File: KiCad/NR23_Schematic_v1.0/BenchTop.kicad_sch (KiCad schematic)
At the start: 13 parts, among them M1 Zero_7R_Motor

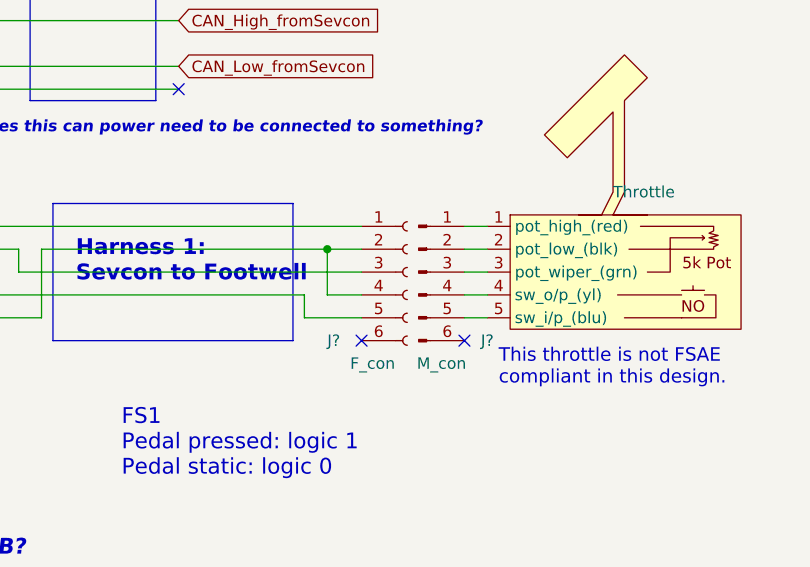
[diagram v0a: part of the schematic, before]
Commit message: Base update (V3)
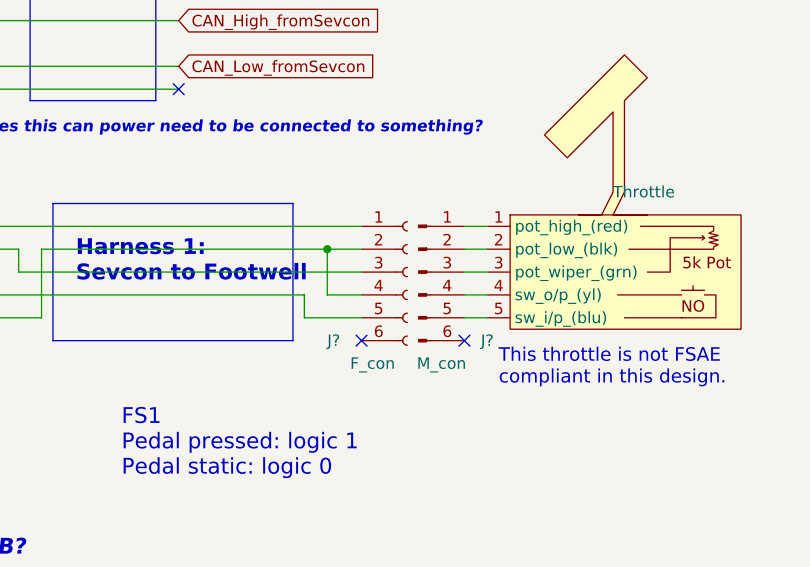
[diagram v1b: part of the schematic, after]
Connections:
- net at U?. (M3): now also J?.2 (Pin_2), J?.4 (Pin_4)
